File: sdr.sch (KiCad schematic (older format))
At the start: 7 parts

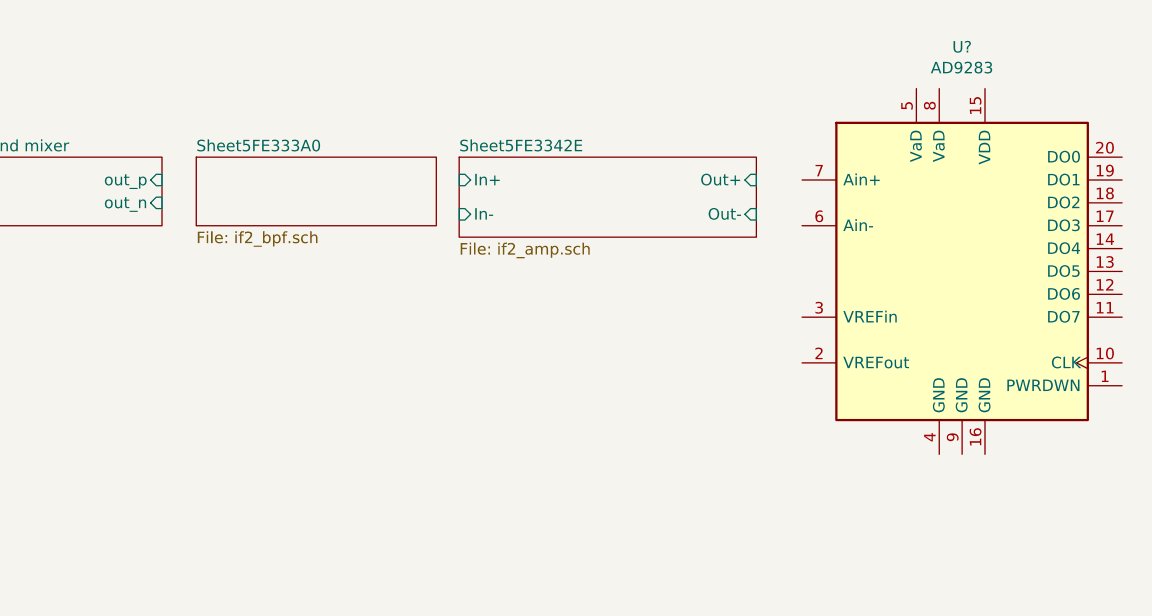
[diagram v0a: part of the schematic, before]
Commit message: if2 completed
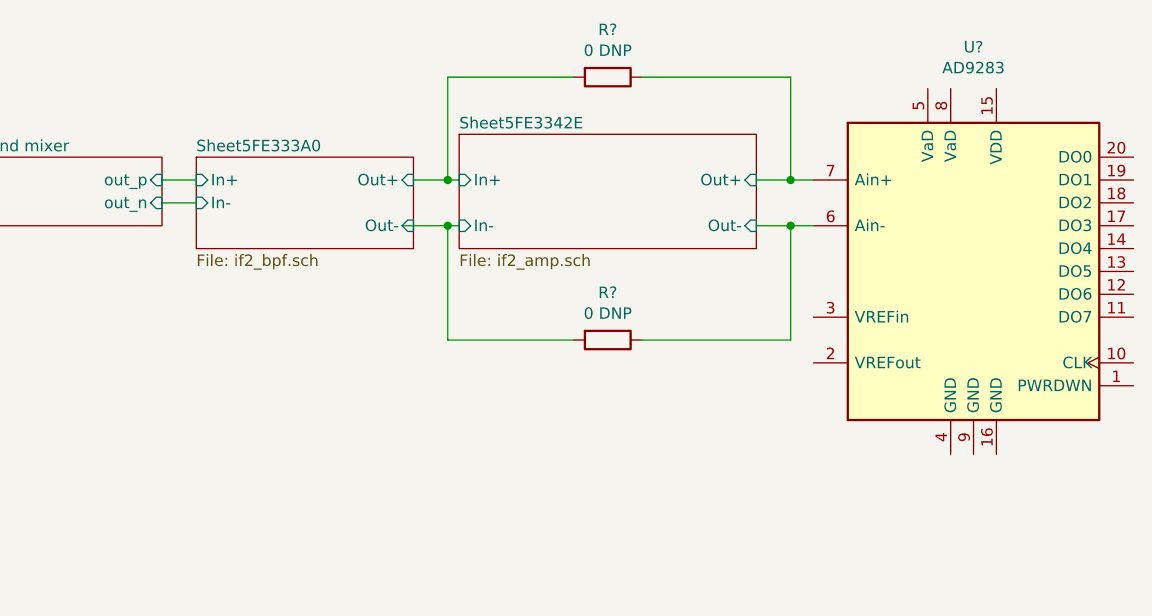
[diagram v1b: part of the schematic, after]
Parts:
- added R? (x2): 0 DNP, symbol Device:R
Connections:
- wire segments 23 -> 41
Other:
- moved on the sheet: U?
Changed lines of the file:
@@
 $EndSheet
 $Sheet
-S 6700 1200 1050 300
+S 6700 1200 950  400
 U 5FE333A1
 F0 "Sheet5FE333A0" 50
 F1 "if2_bpf.sch" 50
+F2 "Out+" I R 7650 1300 50
+F3 "Out-" I R 7650 1500 50
+F4 "In+" I L 6700 1300 50
+F5 "In-" I L 6700 1400 50
 $EndSheet
 $Sheet
-S 7850 1200 1300 350
+S 7850 1100 1300 500
 U 5FE3342F
 F0 "Sheet5FE3342E" 50
 F1 "if2_amp.sch" 50
 F2 "In+" I L 7850 1300 50
-F3 "In-" I L 7850 1450 50
+F3 "In-" I L 7850 1500 50
 F4 "Out+" I R 9150 1300 50
-F5 "Out-" I R 9150 1450 50
+F5 "Out-" I R 9150 1500 50
 $EndSheet
 $Comp
 L Analog_ADC:AD9283 U?
 U 1 1 5FE337CA
-P 10050 1700
-F 0 "U?" H 10050 2681 50  0000 C CNN
-F 1 "AD9283" H 10050 2590 50  0000 C CNN
-F 2 "" H 10050 1700 50  0001 C CNN
-F 3 "https://www.analog.com/media/en/technical-documentation/data-sheets/AD9283.pdf" H 10050 1700 50  0001 C CNN
-	1    10050 1700
+P 10100 1700
+F 0 "U?" H 10100 2681 50  0000 C CNN
+F 1 "AD9283" H 10100 2590 50  0000 C CNN
+F 2 "" H 10100 1700 50  0001 C CNN
+F 3 "https://www.analog.com/media/en/technical-documentation/data-sheets/AD9283.pdf" H 10100 1700 50  0001 C CNN
+	1    10100 1700
 	1    0    0    -1
 $EndComp
@@
 Text Notes 4650 1800 0    50   ~ 0
 Switchable bga2866??
+$Comp
+L Device:R R?
+U 1 1 5FEA317B
+P 8500 850
+F 0 "R?" V 8293 850 50  0000 C CNN
+F 1 "0 DNP" V 8384 850 50  0000 C CNN
+F 2 "" V 8430 850 50  0001 C CNN
+F 3 "~" H 8500 850 50  0001 C CNN
+	1    8500 850
+	0    1    1    0
+$EndComp
+$Comp
+L Device:R R?
+U 1 1 5FEA3DAB
+P 8500 2000
+F 0 "R?" V 8293 2000 50  0000 C CNN
+F 1 "0 DNP" V 8384 2000 50  0000 C CNN
+F 2 "" V 8430 2000 50  0001 C CNN
+F 3 "~" H 8500 2000 50  0001 C CNN
+	1    8500 2000
+	0    1    1    0
+$EndComp
+Wire Wire Line
+	7850 1300 7800 1300
+Wire Wire Line
+	7800 1300 7800 850
+Wire Wire Line
+	7800 850  8350 850
+Wire Wire Line
+	8650 850  9300 850
+Wire Wire Line
+	9300 850  9300 1300
+Wire Wire Line
+	9150 1300 9300 1300
+Wire Wire Line
+	9300 1500 9150 1500
+Wire Wire Line
+	9400 1500 9300 1500
+Connection ~ 9300 1500
+Wire Wire Line
+	9400 1300 9300 1300
+Connection ~ 9300 1300
+Wire Wire Line
+	9300 2000 8650 2000
+Wire Wire Line
+	9300 1500 9300 2000
+Wire Wire Line
+	7800 1500 7800 2000
+Wire Wire Line
+	7800 2000 8350 2000
+Wire Wire Line
+	7650 1300 7800 1300
+Connection ~ 7800 1300
+Wire Wire Line
+	7600 1500 7800 1500
+Connection ~ 7800 1500
+Wire Wire Line
+	7800 1500 7850 1500
+Wire Wire Line
+	6700 1300 6550 1300
+Wire Wire Line
+	6550 1400 6700 1400
 $EndSCHEMATC
